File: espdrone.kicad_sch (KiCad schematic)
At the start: 47 parts, among them U2 USBLC6-2P6, U3 W25Q128JVP, U7 GT-USB-7079C, Y1 Crystal_GND24

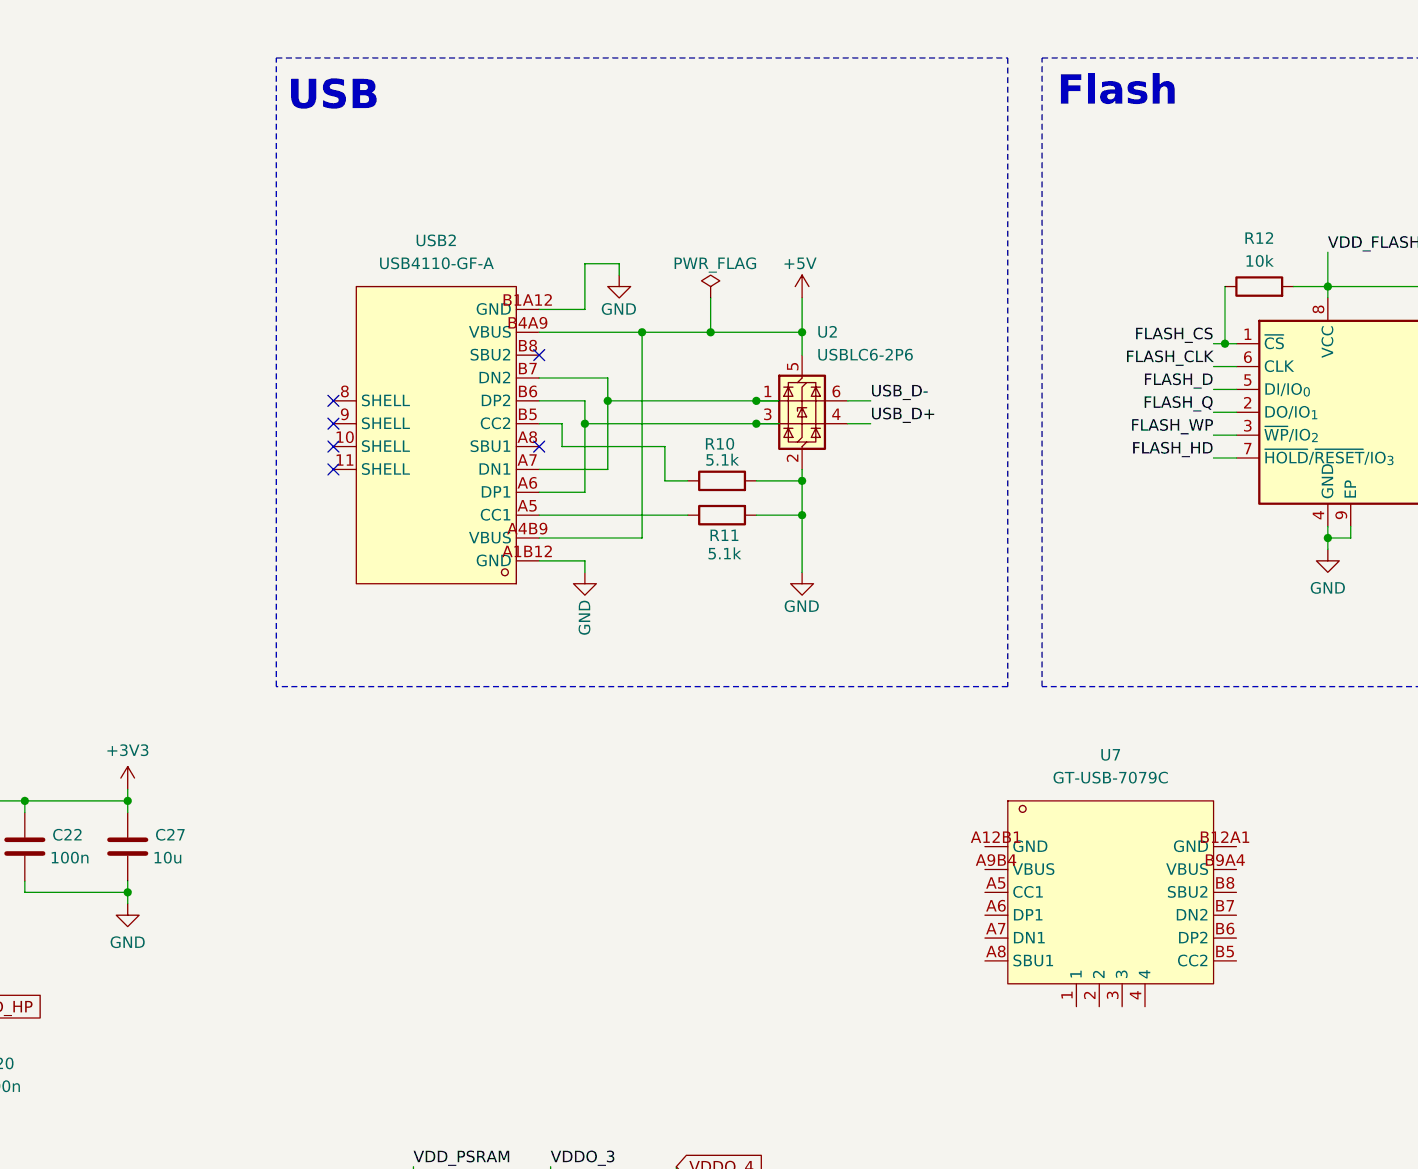
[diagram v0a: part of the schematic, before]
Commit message: Good placement of most FC components
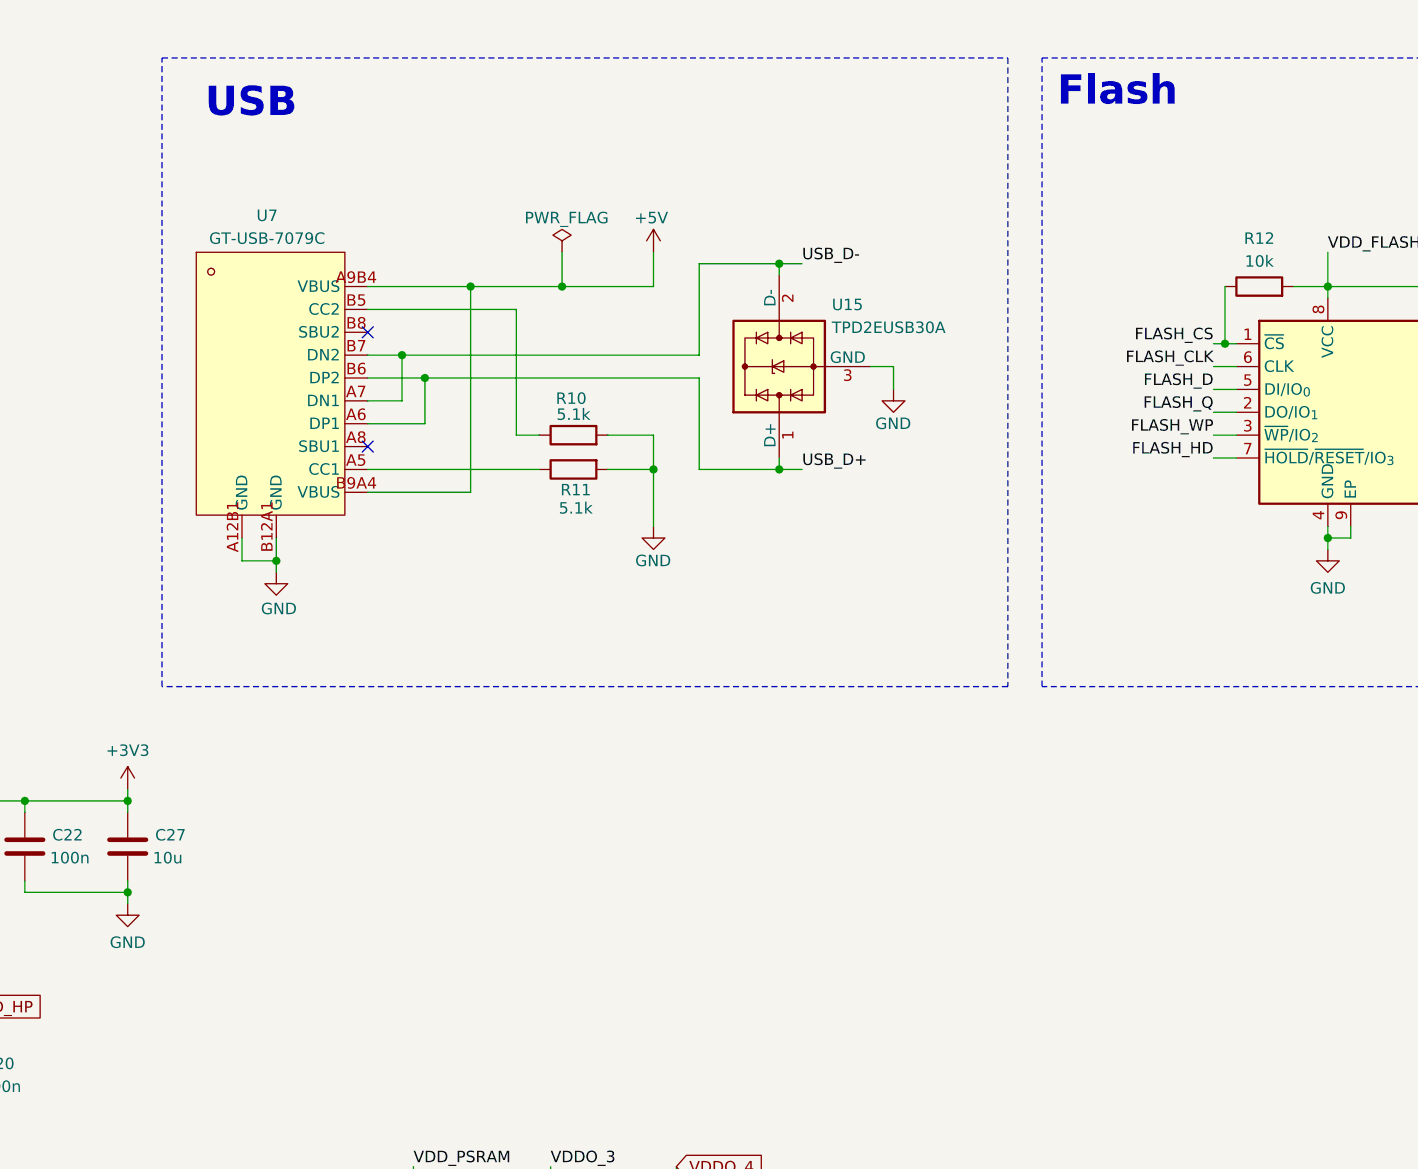
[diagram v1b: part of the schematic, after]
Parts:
- removed U2: USBLC6-2P6, Package_TO_SOT_SMD:SOT-666, symbol Power_Protection:USBLC6-2P6
- removed USB2: USB4110-GF-A, easyeda2kicad:USB-C-SMD_TYPE-C-16P-USB4110-GF-A, symbol easyeda2kicad:USB4110-GF-A
- added U15: TPD2EUSB30A, Package_TO_SOT_SMD:Texas_DRT-3, symbol Power_Protection:TPD2EUSB30A
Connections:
- net +5V: now also U7.A9B4 (VBUS), U7.B9A4 (VBUS)
- net GND: now also U7.A12B1 (GND), U7.B12A1 (GND), U15.3 (GND)
- net USB_D+: now also U7.A6 (DP1), U7.B6 (DP2), U15.1 (D+)
- net USB_D-: now also U7.A7 (DN1), U7.B7 (DN2), U15.2 (D-)
- net at R10.1: now also U7.B5 (CC2)
- net at U7.A5 (CC1): now also R11.1
- no-connect marks 44 -> 40
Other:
- moved on the sheet: R10, R11
